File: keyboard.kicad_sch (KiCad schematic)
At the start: 68 parts, among them J1 Conn_01x06_Socket, J3 Conn_01x02_Socket, SW1 SW_Push, SW10 SW_Push, SW11 SW_Push, SW12 SW_Push, SW13 SW_Push, SW14 SW_Push, SW15 SW_Push, SW16 SW_Push, SW17 SW_Push, SW18 SW_Push, SW19 SW_Push, SW2 SW_Push, SW20 SW_Push, SW21 SW_Push, SW22 SW_Push, SW23 SW_Push, SW24 SW_Push, SW25 SW_Push, SW26 SW_Push, SW27 SW_Push, SW28 SW_Push, SW29 SW_Push, SW3 SW_Push, SW30 SW_Push, SW4 SW_Push, SW5 SW_Push, SW6 SW_Push, SW7 SW_Push, SW8 SW_Push, SW9 SW_Push, U1 rp2040-zero

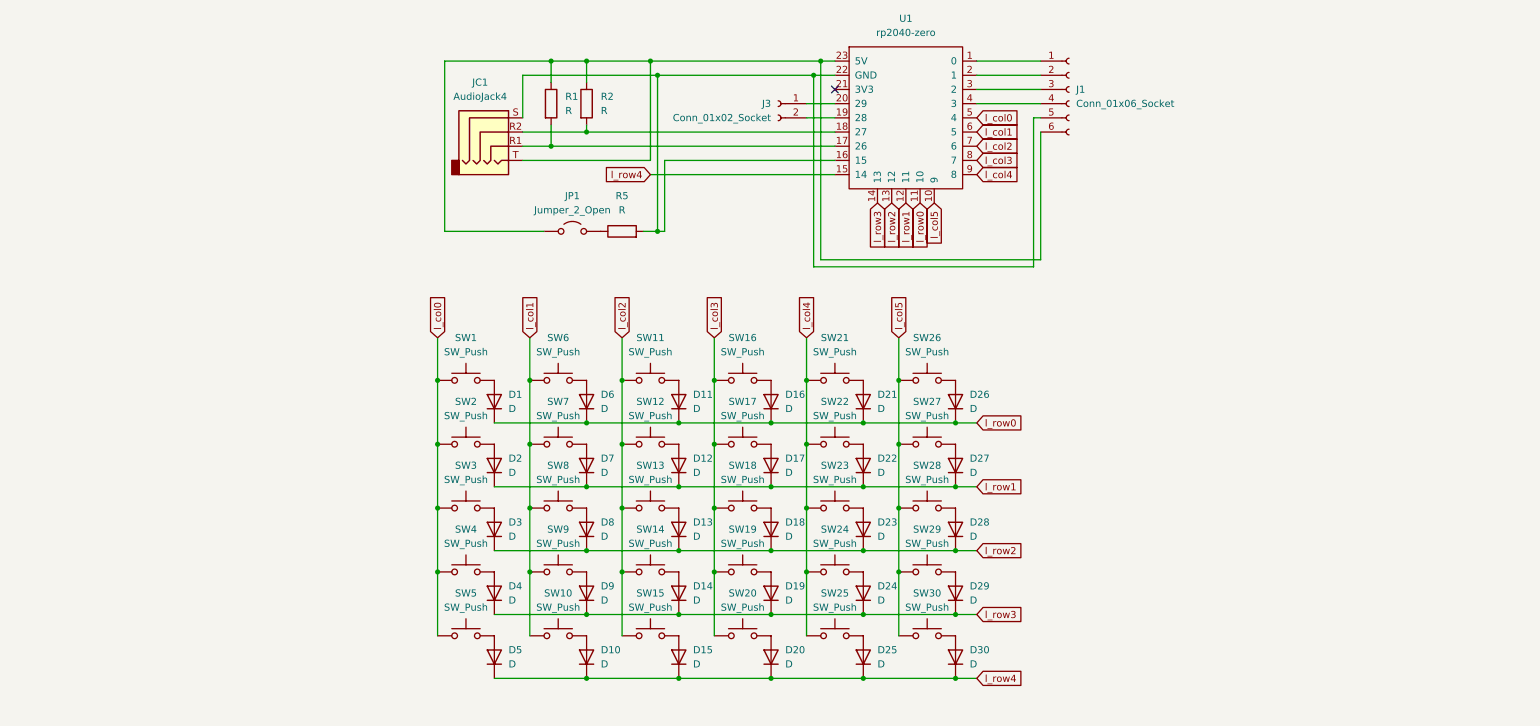
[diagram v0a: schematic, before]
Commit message: wip
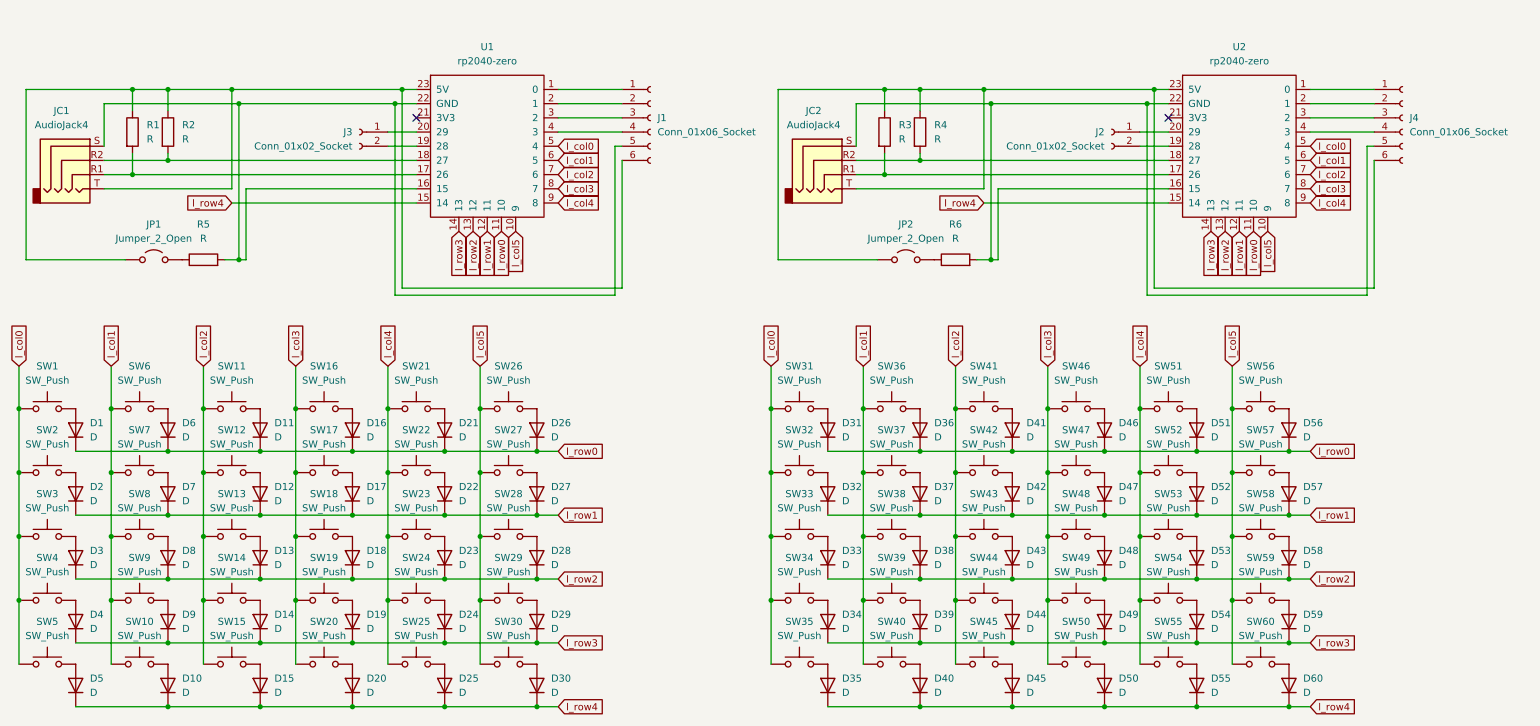
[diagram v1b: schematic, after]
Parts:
- added D31, D32, D33, D34, D35, D36, D37, D38, D39, D40, D41, D42, D43, D44, D45, D46, D47, D48, D49, D50, D51, D52, D53, D54, D55, D56, D57, D58, D59, D60: D, Diode_SMD:D_1206_3216Metric_Pad1.42x1.75mm_HandSolder, symbol Device:D
- added J2: Conn_01x02_Socket, Connector_PinHeader_2.54mm:PinHeader_1x02_P2.54mm_Vertical, symbol Connector:Conn_01x02_Socket
- added J4: Conn_01x06_Socket, Connector_PinHeader_2.54mm:PinHeader_1x06_P2.54mm_Vertical, symbol Connector:Conn_01x06_Socket
- added JC2: AudioJack4, Connector_Audio:Jack_3.5mm_PJ320E_Horizontal, symbol Connector_Audio:AudioJack4
- added JP2: Jumper_2_Open, Jumper:SolderJumper-2_P1.3mm_Open_Pad1.0x1.5mm, symbol Jumper:Jumper_2_Open
- added R3, R4, R6: R, Resistor_SMD:R_1206_3216Metric_Pad1.30x1.75mm_HandSolder, symbol Device:R
- added SW31, SW32, SW33, SW34, SW35, SW36, SW37, SW38, SW39, SW40, SW41, SW42, SW43, SW44, SW46, SW47, SW48, SW49, SW50, SW51, SW52, SW53, SW54, SW55, SW56, SW57, SW58, SW59, SW60: SW_Push, kbd:keyswitch_cherrymx_hotswap_1u, symbol Switch:SW_Push
- added SW45: SW_Push, kbd:keyswitch_cherrymx_hotswap_2u_vertical, symbol Switch:SW_Push
- added U2: rp2040-zero, mcu:rp2040-zero-tht, symbol mcu:rp2040-zero
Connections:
- net l_col0: now also SW31.1, SW32.1, SW33.1, SW34.1, SW35.1, U2.5 (4)
- net l_col1: now also SW36.1, SW37.1, SW38.1, SW39.1, SW40.1, U2.6 (5)
- net l_col2: now also SW41.1, SW42.1, SW43.1, SW44.1, SW45.1, U2.7 (6)
- net l_col3: now also SW46.1, SW47.1, SW48.1, SW49.1, SW50.1, U2.8 (7)
- net l_col4: now also SW51.1, SW52.1, SW53.1, SW54.1, SW55.1, U2.9 (8)
- net l_col5: now also SW56.1, SW57.1, SW58.1, SW59.1, SW60.1, U2.10 (9)
- net l_row0: now also D31.1 (K), D36.1 (K), D41.1 (K), D46.1 (K), D51.1 (K), D56.1 (K), U2.11 (10)
- net l_row1: now also D32.1 (K), D37.1 (K), D42.1 (K), D47.1 (K), D52.1 (K), D57.1 (K), U2.12 (11)
- net l_row2: now also D33.1 (K), D38.1 (K), D43.1 (K), D48.1 (K), D53.1 (K), D58.1 (K), U2.13 (12)
- net l_row3: now also D34.1 (K), D39.1 (K), D44.1 (K), D49.1 (K), D54.1 (K), D59.1 (K), U2.14 (13)
- net l_row4: now also D35.1 (K), D40.1 (K), D45.1 (K), D50.1 (K), D55.1 (K), D60.1 (K), U2.15 (14)
- new net: D36.2 (A), SW36.2
- new net: D58.2 (A), SW58.2
- new net: D56.2 (A), SW56.2
- new net: D60.2 (A), SW60.2
- new net: D32.2 (A), SW32.2
- new net: JP2.2 (B), R6.1
- new net: J4.5 (Pin_5), JC2.S, R6.2, U2.16 (15), U2.22 (GND)
- new net: JC2.R1, R3.2, U2.17 (26)
- new net: JC2.R2, R4.2, U2.18 (27)
- new net: J4.6 (Pin_6), JC2.T, JP2.1 (A), R3.1, R4.1, U2.23 (5V)
- new net: D35.2 (A), SW35.2
- new net: D55.2 (A), SW55.2
- new net: D42.2 (A), SW42.2
- new net: D51.2 (A), SW51.2
- new net: D41.2 (A), SW41.2
- new net: D38.2 (A), SW38.2
- new net: D57.2 (A), SW57.2
- new net: D49.2 (A), SW49.2
- new net: D47.2 (A), SW47.2
- new net: D34.2 (A), SW34.2
- new net: D48.2 (A), SW48.2
- new net: D37.2 (A), SW37.2
- new net: D59.2 (A), SW59.2
- new net: D46.2 (A), SW46.2
- new net: J4.1 (Pin_1), U2.1 (0)
- new net: J2.2 (Pin_2), U2.19 (28)
- new net: J4.2 (Pin_2), U2.2 (1)
- new net: J2.1 (Pin_1), U2.20 (29)
- new net: J4.3 (Pin_3), U2.3 (2)
- new net: J4.4 (Pin_4), U2.4 (3)
- new net: D52.2 (A), SW52.2
- new net: D53.2 (A), SW53.2
- new net: D45.2 (A), SW45.2
- new net: D44.2 (A), SW44.2
- new net: D43.2 (A), SW43.2
- new net: D33.2 (A), SW33.2
- new net: D40.2 (A), SW40.2
- new net: D31.2 (A), SW31.2
- new net: D50.2 (A), SW50.2
- new net: D39.2 (A), SW39.2
- new net: D54.2 (A), SW54.2
- no-connect marks 1 -> 2
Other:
- moved on the sheet: D1, D10, D11, D12, D13, D14, D15, D16, D17, D18, D19, D2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
